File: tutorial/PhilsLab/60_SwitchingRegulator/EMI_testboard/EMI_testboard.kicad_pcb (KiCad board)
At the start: 2 copper layers, 19 x 19 mm, 11 parts

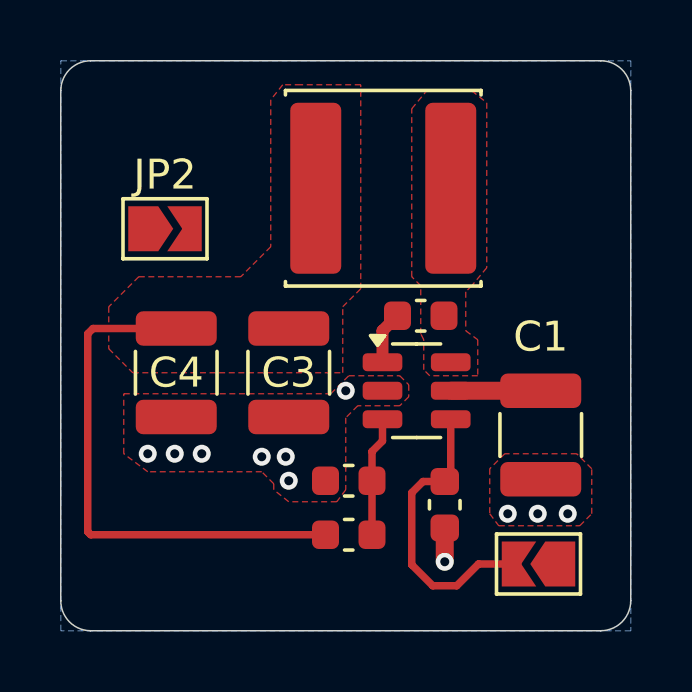
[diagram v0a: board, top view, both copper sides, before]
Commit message: VIDEO #3 :: finished schematic
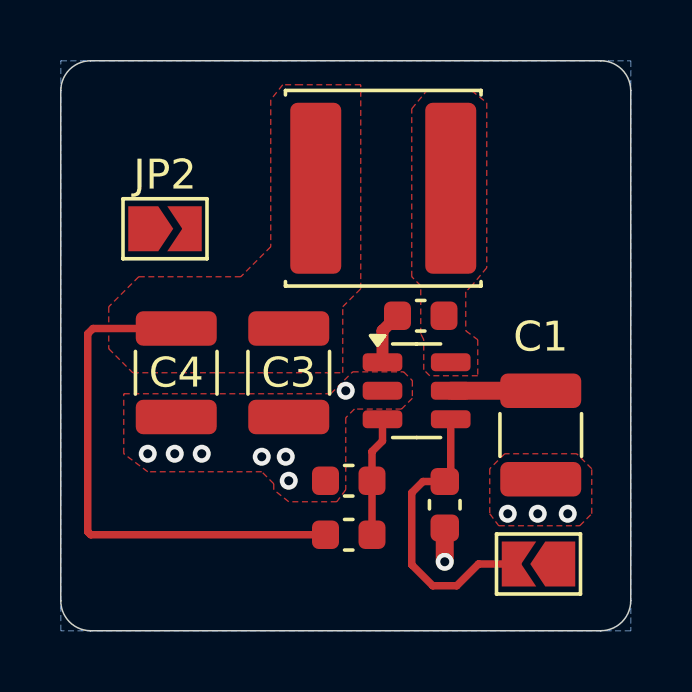
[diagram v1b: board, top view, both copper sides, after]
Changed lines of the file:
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@@
 		(polygon
 			(pts
-				(xy 96.1 69.1) (xy 103 69.1) (xy 103.6 68.5) (xy 105.3 68.5) (xy 105.6 68.8) (xy 105.6 69.2) (xy 105.3 69.5)
-				(xy 103.9 69.5) (xy 103.5 69.9) (xy 103.5 72.3) (xy 103.2 72.7) (xy 101.6 72.7) (xy 101.1 72.3)
-				(xy 101.1 72.1) (xy 100.7 71.7) (xy 96.9 71.7) (xy 96.1 71.1)
+				(xy 96.1 69.1) (xy 103 69.1) (xy 103.73 68.37) (xy 105.43 68.37) (xy 105.72 68.66) (xy 105.72 69.25)
+				(xy 105.36 69.61) (xy 103.79 69.61) (xy 103.5 69.9) (xy 103.5 72.3) (xy 103.2 72.7) (xy 101.6 72.7)
+				(xy 101.1 72.3) (xy 101.1 72.1) (xy 100.7 71.7) (xy 96.9 71.7) (xy 96.1 71.1)
 			)
 		)
